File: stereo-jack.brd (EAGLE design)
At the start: 19 x 51.4 mm, 4 parts, among them J1 STEREOSW

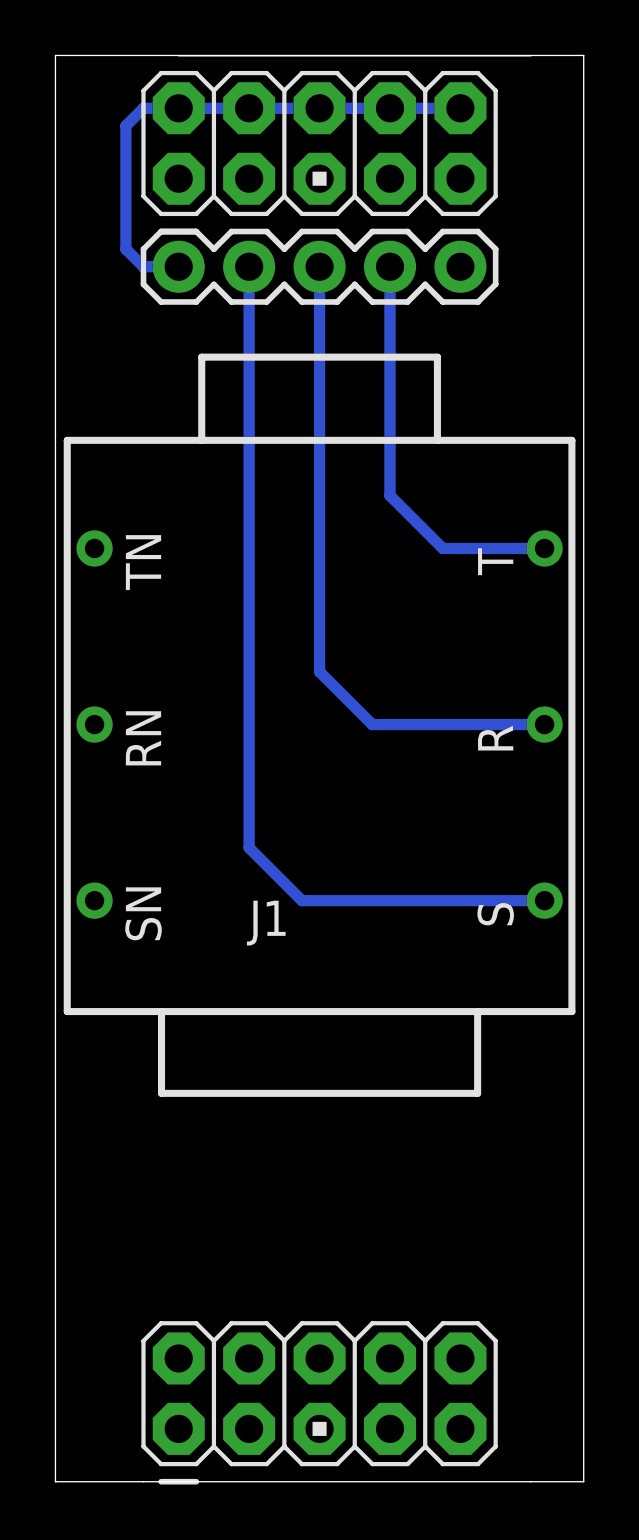
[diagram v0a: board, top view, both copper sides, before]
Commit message: Minor corrections
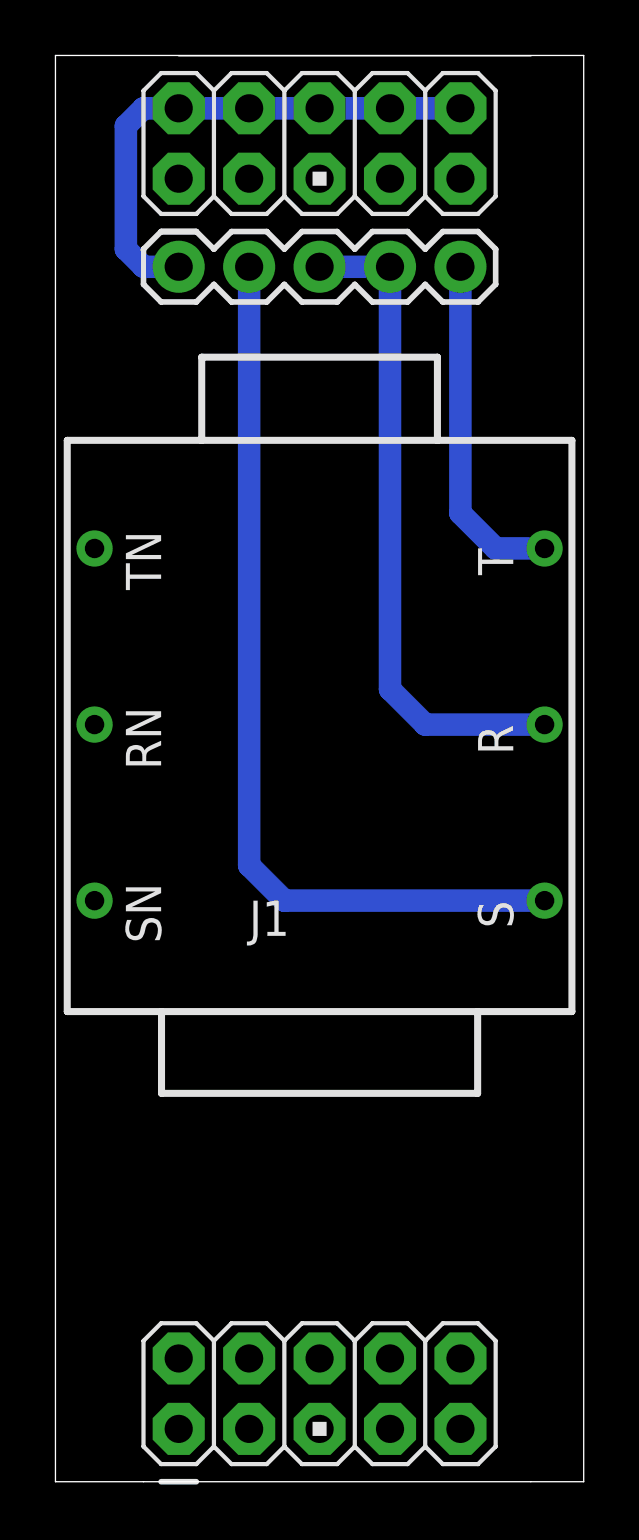
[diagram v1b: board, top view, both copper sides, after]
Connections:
- removed net VEE: JP2.1, JP2.3, JP2.5, JP2.7, JP2.9
- net N$1: no longer J1.SN
- net N$2: now also J1.R, JP3.3; no longer J1.T, J1.TN
- net N$3: now also J1.T, JP3.5; no longer J1.R, J1.RN, JP3.3
- net VCC: now also JP2.1, JP2.3, JP2.5, JP2.7, JP2.9; no longer JP3.5
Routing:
- net VCC: track 0.00 -> 16.8 mm
- net N$3: track 23.5 -> 12.5 mm
- net N$2: track 14.6 -> 23.9 mm
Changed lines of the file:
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@@
 <setting verticaltext="up"/>
 </settings>
-<grid distance="25" unitdist="mil" unit="mm" style="lines" multiple="2" display="yes" altdistance="0.025" altunitdist="inch" altunit="mil"/>
+<grid distance="25" unitdist="mil" unit="mm" style="lines" multiple="2" display="no" altdistance="0.025" altunitdist="inch" altunit="mil"/>
 <layers>
 <layer number="1" name="Top" color="4" fill="1" visible="yes" active="yes"/>
@@
 <contactref element="JP3" pad="1"/>
 <wire x1="37.465" y1="48.26" x2="27.305" y2="48.26" width="0" layer="19" extent="1-16"/>
-<wire x1="27.305" y1="45.085" x2="27.305" y2="48.26" width="0" layer="19" extent="1-16"/>
 <wire x1="32.385" y1="48.26" x2="34.925" y2="48.26" width="0" layer="19" extent="1-1"/>
 <wire x1="29.845" y1="48.26" x2="32.385" y2="48.26" width="0" layer="19" extent="1-1"/>
@@
 <wire x1="34.925" y1="5.715" x2="32.385" y2="5.715" width="0" layer="19" extent="1-1"/>
 <wire x1="37.465" y1="5.715" x2="34.925" y2="5.715" width="0" layer="19" extent="1-1"/>
-<wire x1="27.305" y1="45.085" x2="26.035" y2="45.085" width="0.4064" layer="16"/>
-<wire x1="26.035" y1="45.085" x2="25.4" y2="45.72" width="0.4064" layer="16"/>
 <wire x1="25.4" y1="45.72" x2="25.4" y2="50.165" width="0.4064" layer="16"/>
 <wire x1="25.4" y1="50.165" x2="26.035" y2="50.8" width="0.4064" layer="16"/>
 <wire x1="26.035" y1="50.8" x2="37.465" y2="50.8" width="0.4064" layer="16"/>
 <wire x1="37.465" y1="50.8" x2="37.465" y2="48.26" width="0" layer="19" extent="1-16"/>
+<wire x1="27.305" y1="45.085" x2="26.035" y2="45.085" width="0.8128" layer="16"/>
+<wire x1="26.035" y1="45.085" x2="25.4" y2="45.72" width="0.8128" layer="16"/>
+<wire x1="25.4" y1="45.72" x2="27.305" y2="48.26" width="0" layer="19" extent="1-16"/>
 </signal>
 <signal name="VCC">
@@
 <contactref element="JP1" pad="2"/>
 <contactref element="JP1" pad="10"/>
-<contactref element="JP3" pad="5"/>
-<wire x1="27.305" y1="50.8" x2="37.465" y2="50.8" width="0" layer="19" extent="1-16"/>
-<wire x1="37.465" y1="50.8" x2="38.1" y2="50.8" width="0" layer="19" extent="1-16"/>
-<wire x1="38.1" y1="50.8" x2="40.005" y2="48.895" width="0" layer="19" extent="1-16"/>
-<wire x1="37.465" y1="45.085" x2="38.1" y2="45.085" width="0" layer="19" extent="1-16"/>
-<wire x1="38.1" y1="45.085" x2="40.005" y2="46.99" width="0" layer="19" extent="1-16"/>
-<wire x1="40.005" y1="46.99" x2="40.005" y2="48.895" width="0" layer="19" extent="1-16"/>
-<wire x1="32.385" y1="50.8" x2="34.925" y2="50.8" width="0" layer="19" extent="1-1"/>
-<wire x1="29.845" y1="50.8" x2="32.385" y2="50.8" width="0" layer="19" extent="1-1"/>
-<wire x1="37.465" y1="50.8" x2="34.925" y2="50.8" width="0" layer="19" extent="1-1"/>
-</signal>
-<signal name="VEE">
 <contactref element="JP2" pad="7"/>
 <contactref element="JP2" pad="5"/>
@@
 <contactref element="JP2" pad="1"/>
 <contactref element="JP2" pad="9"/>
-<wire x1="37.465" y1="3.175" x2="29.845" y2="3.175" width="0" layer="19" extent="1-16"/>
-<wire x1="29.845" y1="3.175" x2="27.305" y2="3.175" width="0" layer="19" extent="1-16"/>
-<wire x1="32.385" y1="3.175" x2="34.925" y2="3.175" width="0" layer="19" extent="1-1"/>
+<wire x1="37.465" y1="50.8" x2="26.035" y2="50.8" width="0.8128" layer="16"/>
+<wire x1="26.035" y1="50.8" x2="25.4" y2="50.165" width="0.8128" layer="16"/>
+<wire x1="25.4" y1="50.165" x2="25.4" y2="45.72" width="0.8128" layer="16"/>
+<wire x1="32.385" y1="50.8" x2="34.925" y2="50.8" width="0" layer="19" extent="1-1"/>
+<wire x1="29.845" y1="50.8" x2="32.385" y2="50.8" width="0" layer="19" extent="1-1"/>
+<wire x1="27.305" y1="50.8" x2="29.845" y2="50.8" width="0" layer="19" extent="1-1"/>
+<wire x1="26.035" y1="50.8" x2="27.305" y2="50.8" width="0" layer="19" extent="16-16"/>
+<wire x1="27.305" y1="3.175" x2="25.4" y2="45.72" width="0" layer="19" extent="16-16"/>
+<wire x1="29.845" y1="3.175" x2="27.305" y2="3.175" width="0" layer="19" extent="1-1"/>
+<wire x1="32.385" y1="3.175" x2="29.845" y2="3.175" width="0" layer="19" extent="1-1"/>
+<wire x1="34.925" y1="3.175" x2="32.385" y2="3.175" width="0" layer="19" extent="1-1"/>
 <wire x1="37.465" y1="3.175" x2="34.925" y2="3.175" width="0" layer="19" extent="1-1"/>
 </signal>
+<signal name="N$1">
+<contactref element="JP3" pad="2"/>
+<contactref element="J1" pad="S"/>
+<wire x1="29.845" y1="45.085" x2="29.845" y2="23.495" width="0.8128" layer="16"/>
+<wire x1="29.845" y1="23.495" x2="31.115" y2="22.225" width="0.8128" layer="16"/>
+<wire x1="31.115" y1="22.225" x2="40.5" y2="22.225" width="0.8128" layer="16"/>
+</signal>
 <signal name="N$2">
-<contactref element="JP3" pad="4"/>
-<wire x1="35.52" y1="8.295" x2="34.925" y2="45.085" width="0" layer="19" extent="1-16"/>
-<contactref element="J1" pad="T"/>
-<contactref element="J1" pad="TN"/>
-<wire x1="24.27" y1="34.925" x2="40.5" y2="34.925" width="0" layer="19" extent="1-1"/>
-<wire x1="40.5" y1="34.925" x2="36.83" y2="34.925" width="0.4064" layer="16"/>
-<wire x1="36.83" y1="34.925" x2="34.925" y2="36.83" width="0.4064" layer="16"/>
-<wire x1="34.925" y1="36.83" x2="34.925" y2="45.085" width="0.4064" layer="16"/>
-</signal>
-<signal name="N$3">
 <contactref element="JP3" pad="3"/>
 <contactref element="J1" pad="R"/>
-<contactref element="J1" pad="RN"/>
-<wire x1="40.5" y1="28.575" x2="34.29" y2="28.575" width="0.4064" layer="16"/>
-<wire x1="34.29" y1="28.575" x2="32.385" y2="30.48" width="0.4064" layer="16"/>
-<wire x1="32.385" y1="30.48" x2="32.385" y2="45.085" width="0.4064" layer="16"/>
-<wire x1="24.27" y1="28.575" x2="32.385" y2="30.48" width="0" layer="19" extent="16-16"/>
-</signal>
-<signal name="N$1">
-<contactref element="JP3" pad="2"/>
-<contactref element="J1" pad="SN"/>
-<contactref element="J1" pad="S"/>
-<wire x1="40.5" y1="22.225" x2="31.75" y2="22.225" width="0.4064" layer="16"/>
-<wire x1="31.75" y1="22.225" x2="29.845" y2="24.13" width="0.4064" layer="16"/>
-<wire x1="29.845" y1="24.13" x2="29.845" y2="45.085" width="0.4064" layer="16"/>
-<wire x1="24.27" y1="22.225" x2="29.845" y2="24.13" width="0" layer="19" extent="16-16"/>
+<contactref element="JP3" pad="4"/>
+<wire x1="32.385" y1="45.085" x2="34.925" y2="45.085" width="0.8128" layer="16"/>
+<wire x1="34.925" y1="45.085" x2="34.925" y2="29.845" width="0.8128" layer="16"/>
+<wire x1="34.925" y1="29.845" x2="36.195" y2="28.575" width="0.8128" layer="16"/>
+<wire x1="36.195" y1="28.575" x2="40.5" y2="28.575" width="0.8128" layer="16"/>
+</signal>
+<signal name="N$3">
+<contactref element="JP3" pad="5"/>
+<contactref element="J1" pad="T"/>
+<wire x1="40.5" y1="34.925" x2="38.735" y2="34.925" width="0.8128" layer="16"/>
+<wire x1="38.735" y1="34.925" x2="37.465" y2="36.195" width="0.8128" layer="16"/>
+<wire x1="37.465" y1="36.195" x2="37.465" y2="45.085" width="0.8128" layer="16"/>
 </signal>
 </signals>
